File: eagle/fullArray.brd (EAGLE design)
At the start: 40 x 64 mm, 117 parts

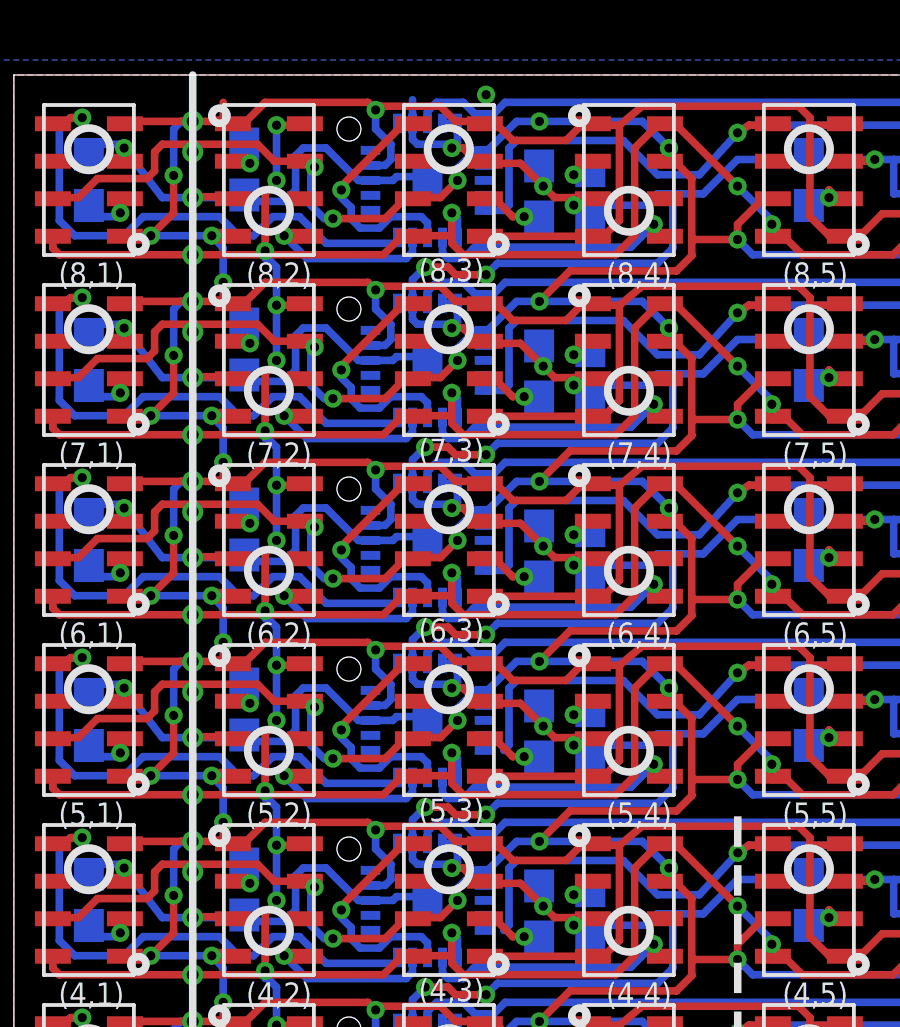
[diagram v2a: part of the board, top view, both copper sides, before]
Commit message: now with proper address pin configurations
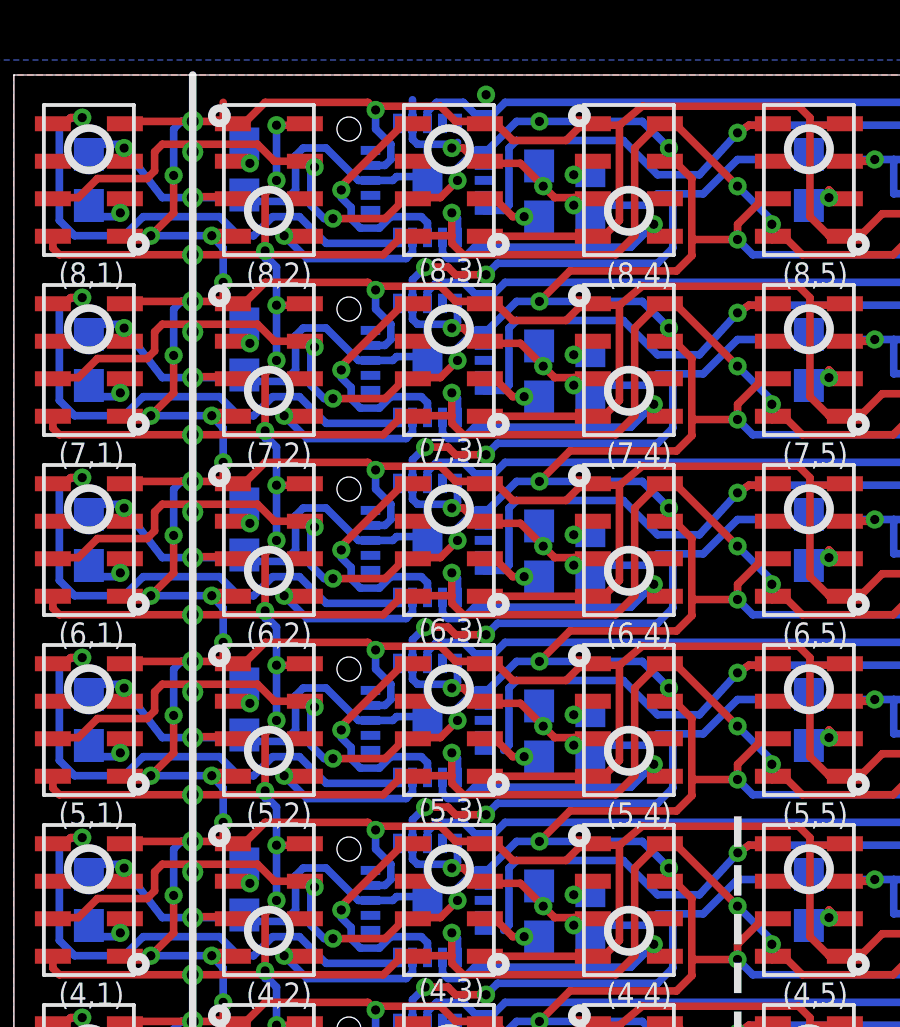
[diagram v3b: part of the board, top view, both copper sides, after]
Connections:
- net ADDR00 renamed ADDR1
- removed net ADDR01: AT2.11
- removed net ADDR02: AT3.11
- removed net ADDR03: AT4.11
- removed net ADDR04: AT5.11
- removed net ADDR05: AT6.11
- removed net ADDR06: AT7.11
- removed net ADDR07: AT8.11
- new net ADDR2: AT2.12
- new net ADDR3: AT3.11, AT3.12
- new net ADDR4: AT4.14
- new net ADDR5: AT5.11, AT5.14
- new net ADDR6: AT6.12, AT6.14
- new net ADDR7: AT7.11, AT7.12, AT7.14
- new net ADDR8: AT8.15
- net GND: now also AT2.11, AT4.11, AT6.11, AT8.11; no longer AT2.12, AT3.12, AT4.14, AT5.14, AT6.12, AT6.14, AT7.12, AT7.14, AT8.15
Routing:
- net GND: track 503.1 -> 500.0 mm
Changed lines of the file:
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@@
 <contactref element="C5" pad="2"/>
 <contactref element="AT2" pad="15"/>
-<contactref element="AT2" pad="12"/>
 <contactref element="AT2" pad="14"/>
 <wire x1="-5.213" y1="26.386" x2="-5.713" y2="26.386" width="0.254" layer="16"/>
@@
 <contactref element="C13" pad="2"/>
 <contactref element="AT3" pad="15"/>
-<contactref element="AT3" pad="12"/>
 <contactref element="AT3" pad="14"/>
 <wire x1="-5.213" y1="32.386" x2="-5.713" y2="32.386" width="0.254" layer="16"/>
@@
 <contactref element="AT4" pad="15"/>
 <contactref element="AT4" pad="12"/>
-<contactref element="AT4" pad="14"/>
-<wire x1="-5.213" y1="38.386" x2="-5.713" y2="38.386" width="0.254" layer="16"/>
 <wire x1="-4.3" y1="37.125" x2="-4.242" y2="37.183" width="0.254" layer="1"/>
 <wire x1="-4.202" y1="37.125" x2="-4.133" y2="37.056" width="0.254" layer="1"/>
@@
 <contactref element="AT5" pad="15"/>
 <contactref element="AT5" pad="12"/>
-<contactref element="AT5" pad="14"/>
-<wire x1="-5.213" y1="44.386" x2="-5.713" y2="44.386" width="0.254" layer="16"/>
 <wire x1="-4.3" y1="43.125" x2="-4.242" y2="43.183" width="0.254" layer="1"/>
 <wire x1="-4.202" y1="43.125" x2="-4.133" y2="43.056" width="0.254" layer="1"/>
@@
 <contactref element="C28" pad="2"/>
 <contactref element="AT6" pad="15"/>
-<contactref element="AT6" pad="12"/>
-<contactref element="AT6" pad="14"/>
-<wire x1="-5.213" y1="50.386" x2="-5.713" y2="50.386" width="0.254" layer="16"/>
 <wire x1="-4.3" y1="49.125" x2="-4.242" y2="49.183" width="0.254" layer="1"/>
 <wire x1="-4.202" y1="49.125" x2="-4.133" y2="49.056" width="0.254" layer="1"/>
@@
 <contactref element="C33" pad="2"/>
 <contactref element="AT7" pad="15"/>
-<contactref element="AT7" pad="12"/>
-<contactref element="AT7" pad="14"/>
-<wire x1="-5.213" y1="56.386" x2="-5.713" y2="56.386" width="0.254" layer="16"/>
 <wire x1="-4.3" y1="55.125" x2="-4.242" y2="55.183" width="0.254" layer="1"/>
 <wire x1="-4.202" y1="55.125" x2="-4.133" y2="55.056" width="0.254" layer="1"/>
@@
 <contactref element="(8,1)" pad="3"/>
 <contactref element="C38" pad="2"/>
-<contactref element="AT8" pad="15"/>
 <contactref element="AT8" pad="12"/>
-<contactref element="AT8" pad="14"/>
-<wire x1="-5.213" y1="62.386" x2="-5.713" y2="62.386" width="0.254" layer="16"/>
 <wire x1="-4.3" y1="61.125" x2="-4.242" y2="61.183" width="0.254" layer="1"/>
 <wire x1="-4.202" y1="61.125" x2="-4.133" y2="61.056" width="0.254" layer="1"/>
@@
 <wire x1="-5.276" y1="61.691" x2="-5.403" y2="61.564" width="0.254" layer="16"/>
 <wire x1="-5.403" y1="61.564" x2="-5.213" y2="61.754" width="0.254" layer="16"/>
-<wire x1="-5.213" y1="61.754" x2="-5.213" y2="62.386" width="0.254" layer="16"/>
 <wire x1="-17.5" y1="61.35" x2="-17.341" y2="61.509" width="0.254" layer="16"/>
 <wire x1="-17.341" y1="61.509" x2="-17.341" y2="61.564" width="0.254" layer="16"/>
@@
 </polygon>
 <via x="10" y="12.5" extent="1-16" drill="0.475" shape="octagon"/>
+<contactref element="AT8" pad="11"/>
+<contactref element="AT8" pad="14"/>
+<contactref element="AT6" pad="11"/>
+<contactref element="AT4" pad="11"/>
+<contactref element="AT2" pad="11"/>
+<wire x1="-5.713" y1="62.386" x2="-4.26" y2="63.342" width="0" layer="19" extent="16-16"/>
+<wire x1="-5.213" y1="61.754" x2="-5.713" y2="62.386" width="0" layer="19" extent="16-16"/>
+<wire x1="1.963" y1="59.882" x2="1.963" y2="60.04" width="0" layer="19" extent="16-16"/>
+<wire x1="1.963" y1="53.882" x2="1.963" y2="54.04" width="0" layer="19" extent="16-16"/>
+<wire x1="1.963" y1="47.882" x2="1.963" y2="48.04" width="0" layer="19" extent="16-16"/>
+<wire x1="1.963" y1="41.882" x2="1.963" y2="42.04" width="0" layer="19" extent="16-16"/>
+<wire x1="1.963" y1="35.882" x2="1.963" y2="36.04" width="0" layer="19" extent="16-16"/>
+<wire x1="1.963" y1="29.882" x2="1.963" y2="30.04" width="0" layer="19" extent="16-16"/>
+<wire x1="1.963" y1="23.882" x2="1.963" y2="24.04" width="0" layer="19" extent="16-16"/>
+<wire x1="-6.713" y1="62.386" x2="-6.713" y2="61.858" width="0" layer="19" extent="16-16"/>
+<wire x1="-7.213" y1="62.386" x2="-6.713" y2="62.386" width="0" layer="19" extent="16-16"/>
+<wire x1="-6.713" y1="44.386" x2="-6.713" y2="43.858" width="0" layer="19" extent="16-16"/>
+<wire x1="-6.713" y1="38.386" x2="-6.713" y2="37.858" width="0" layer="19" extent="16-16"/>
+<wire x1="-7.213" y1="38.386" x2="-6.713" y2="38.386" width="0" layer="19" extent="16-16"/>
+<wire x1="-6.713" y1="20.386" x2="-6.713" y2="19.858" width="0" layer="19" extent="16-16"/>
+<wire x1="-7.213" y1="50.386" x2="-6.713" y2="49.858" width="0" layer="19" extent="16-16"/>
+<wire x1="-7.213" y1="26.386" x2="-6.713" y2="25.858" width="0" layer="19" extent="16-16"/>
+<wire x1="1" y1="13.5" x2="-0.784" y2="17.111" width="0" layer="19" extent="16-16"/>
+<wire x1="-0.5" y1="12.5" x2="1" y2="13.5" width="0" layer="19" extent="1-1"/>
+<wire x1="-1" y1="7.5" x2="-1" y2="11.4" width="0" layer="19" extent="1-1"/>
+<wire x1="6" y1="7.75" x2="3.4" y2="7.5" width="0" layer="19" extent="1-1"/>
+<wire x1="10" y1="12.5" x2="12.552" y2="17.23" width="0" layer="19" extent="1-1"/>
+<wire x1="-8.55" y1="10.05" x2="-3.4" y2="7.5" width="0" layer="19" extent="1-1"/>
+<wire x1="-14.15" y1="10.25" x2="-8.55" y2="10.05" width="0" layer="19" extent="1-1"/>
+<wire x1="-14.15" y1="8.25" x2="-14.15" y2="10.25" width="0" layer="19" extent="1-1"/>
+<wire x1="-14.15" y1="6.25" x2="-14.15" y2="8.25" width="0" layer="19" extent="1-1"/>
+<wire x1="-9.2" y1="4.175" x2="-14.15" y2="6.25" width="0" layer="19" extent="1-1"/>
+<wire x1="6.84" y1="1.5" x2="6" y2="7.75" width="0" layer="19" extent="1-1"/>
+<wire x1="12.96" y1="6.73" x2="10" y2="12.5" width="0" layer="19" extent="1-1"/>
 </signal>
 <signal name="3.3V">
@@
 <wire x1="-3.625" y1="21.088" x2="11.615" y2="21.088" width="0.254" layer="16"/>
 </signal>
-<signal name="ADDR00">
+<signal name="ADDR1">
 <contactref element="AT1" pad="11"/>
 </signal>
@@
 <wire x1="-3.625" y1="27.088" x2="11.615" y2="27.088" width="0.254" layer="16"/>
 </signal>
-<signal name="ADDR01">
-<contactref element="AT2" pad="11"/>
-</signal>
 <signal name="CAP06">
 <contactref element="C15" pad="1"/>
@@
 <wire x1="-3.625" y1="33.088" x2="11.615" y2="33.088" width="0.254" layer="16"/>
 </signal>
-<signal name="ADDR02">
+<signal name="ADDR3">
 <contactref element="AT3" pad="11"/>
+<contactref element="AT3" pad="12"/>
+<wire x1="-6.713" y1="32.386" x2="-7.213" y2="32.386" width="0" layer="19" extent="16-16"/>
 </signal>
 <signal name="CAP12">
@@
 <wire x1="-12.057" y1="37.437" x2="-12.32" y2="37.7" width="0.254" layer="16"/>
 </signal>
-<signal name="ADDR03">
-<contactref element="AT4" pad="11"/>
-</signal>
 <signal name="CAP17">
 <contactref element="C25" pad="1"/>
@@
 <wire x1="-3.625" y1="45.088" x2="11.615" y2="45.088" width="0.254" layer="16"/>
 </signal>
-<signal name="ADDR04">
+<signal name="ADDR5">
 <contactref element="AT5" pad="11"/>
+<contactref element="AT5" pad="14"/>
+<wire x1="-5.713" y1="44.386" x2="-7.213" y2="44.386" width="0" layer="19" extent="16-16"/>
 </signal>
 <signal name="CAP23">
@@
 <wire x1="-3.625" y1="51.088" x2="11.615" y2="51.088" width="0.254" layer="16"/>
 </signal>
-<signal name="ADDR05">
-<contactref element="AT6" pad="11"/>
-</signal>
 <signal name="CAP28">
 <contactref element="C35" pad="1"/>
@@
 <wire x1="9.995" y1="56.357" x2="10" y2="56.357" width="0.254" layer="16"/>
 </signal>
-<signal name="ADDR06">
+<signal name="ADDR7">
 <contactref element="AT7" pad="11"/>
+<contactref element="AT7" pad="12"/>
+<contactref element="AT7" pad="14"/>
+<wire x1="-6.713" y1="56.386" x2="-7.213" y2="56.386" width="0" layer="19" extent="16-16"/>
+<wire x1="-5.713" y1="56.386" x2="-6.713" y2="56.386" width="0" layer="19" extent="16-16"/>
 </signal>
 <signal name="CAP34">
@@
 <wire x1="9.995" y1="62.357" x2="10" y2="62.357" width="0.254" layer="16"/>
 </signal>
-<signal name="ADDR07">
-<contactref element="AT8" pad="11"/>
-</signal>
 <signal name="RST56">
 <contactref element="PROG6" pad="1"/>
@@
 <contactref element="PROG1" pad="5"/>
 </signal>
+<signal name="ADDR8">
+<contactref element="AT8" pad="15"/>
+</signal>
+<signal name="ADDR6">
+<contactref element="AT6" pad="12"/>
+<contactref element="AT6" pad="14"/>
+<wire x1="-5.713" y1="50.386" x2="-6.713" y2="50.386" width="0" layer="19" extent="16-16"/>
+</signal>
+<signal name="ADDR4">
+<contactref element="AT4" pad="14"/>
+</signal>
+<signal name="ADDR2">
+<contactref element="AT2" pad="12"/>
+</signal>
 </signals>
-<errors>
-</errors>
 </board>
 </drawing>

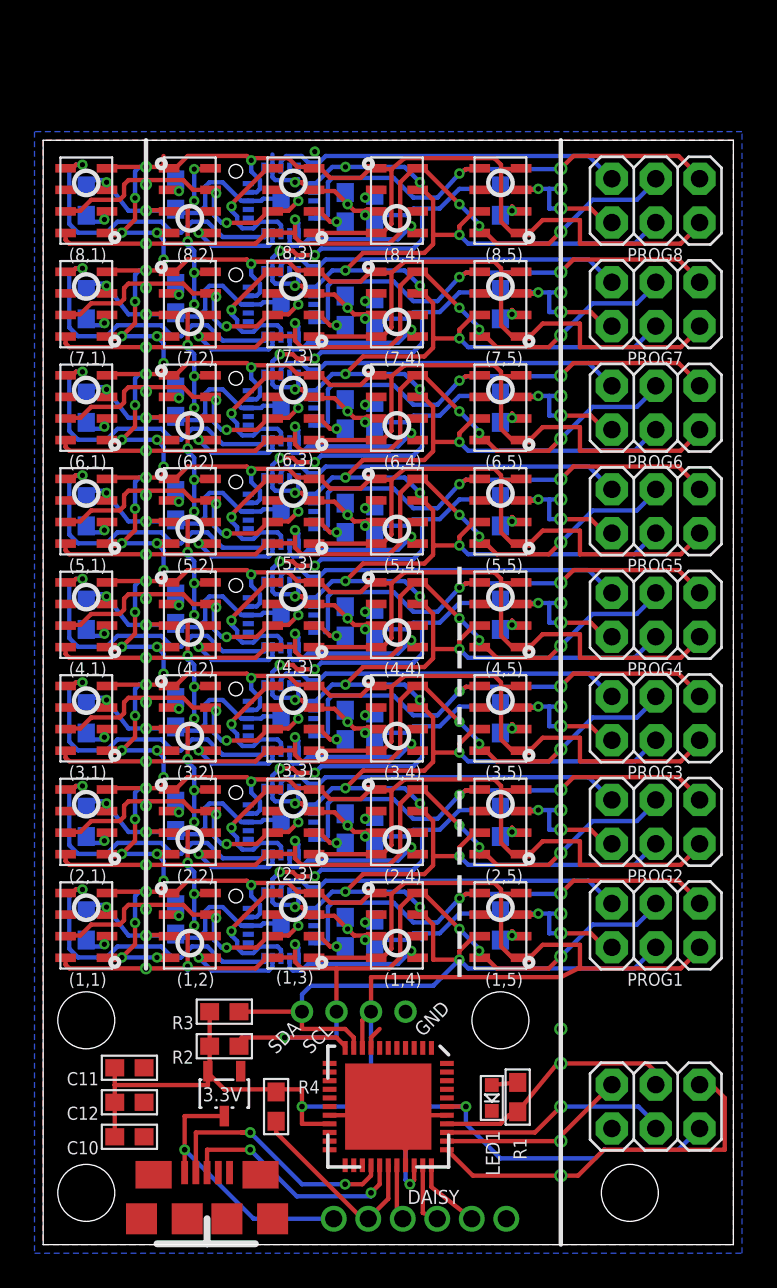
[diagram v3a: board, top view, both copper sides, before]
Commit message: fixed few ERC glitches and ADDR routing
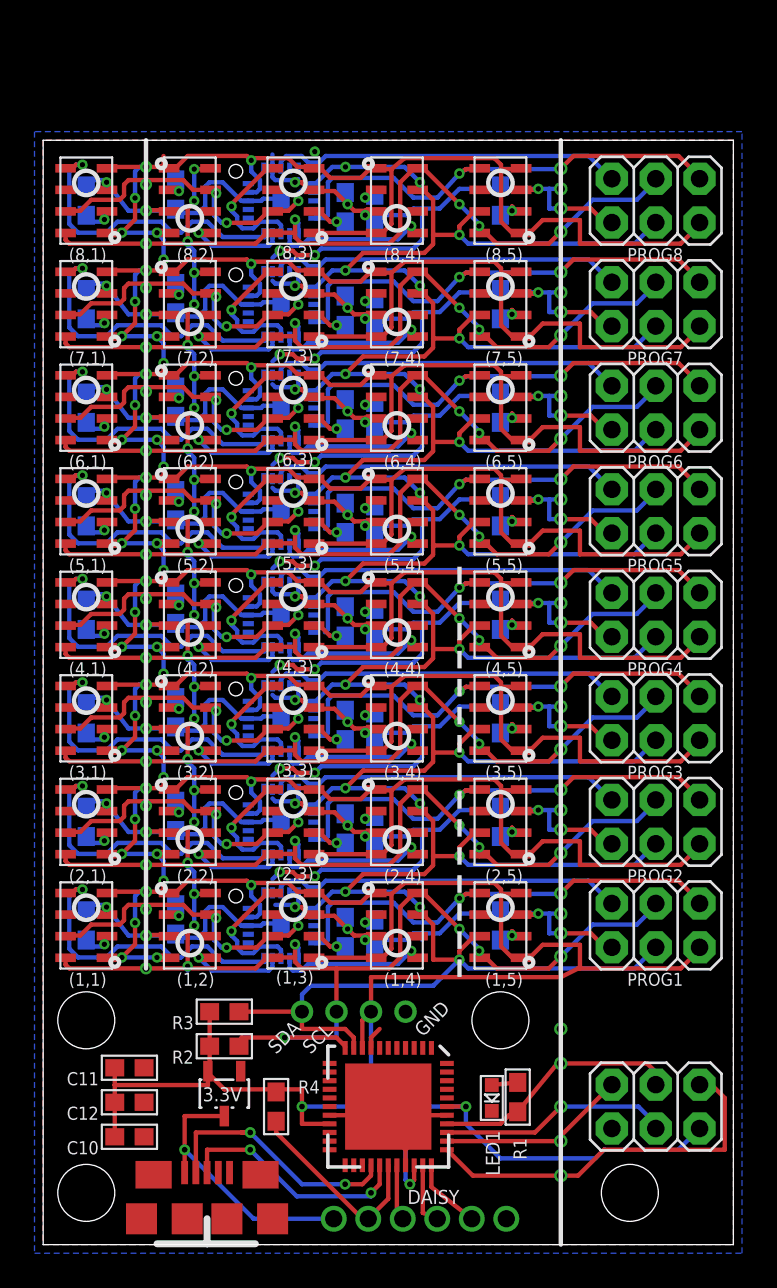
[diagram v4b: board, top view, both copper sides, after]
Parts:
- R1: value (none) -> 120o
- R2, R3: value (none) -> 4.7K
- R4: value (none) -> 4.7k
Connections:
- removed net RESET0: AT1.13
- net RESET1: now also AT1.13
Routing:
- net RESET1: track 0.00 -> 20.5 mm
- net RESET0: track 20.5 -> 0.00 mm
- net GND: track 500.0 -> 491.0 mm
